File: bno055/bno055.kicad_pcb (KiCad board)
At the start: 4 copper layers, 15 parts, among them U1 BNO055, Y1 NX3215SA-32.768K-STD-MUA-14

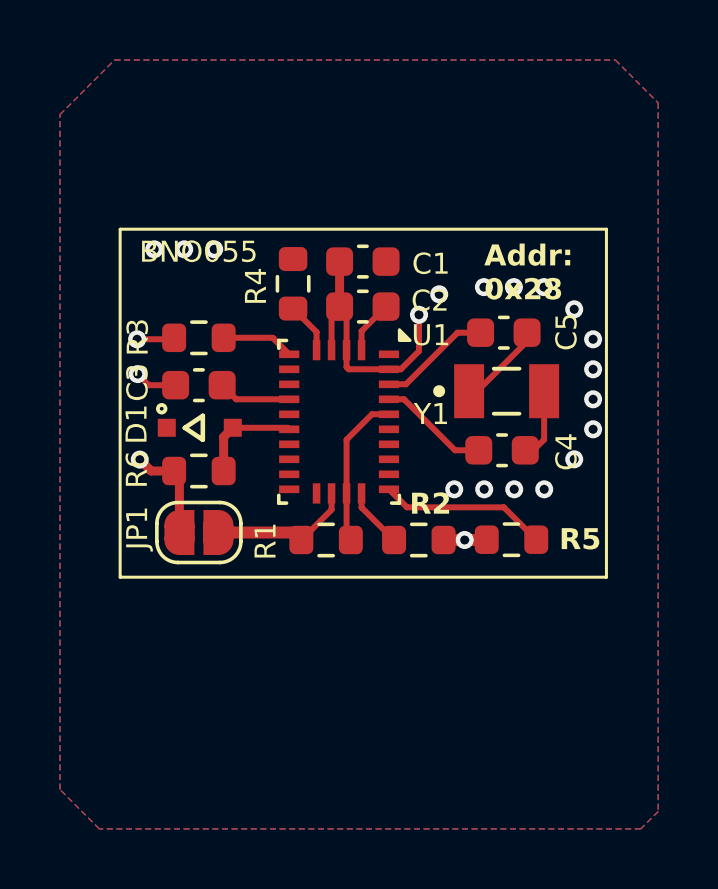
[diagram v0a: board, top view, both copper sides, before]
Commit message: fixed BNO055
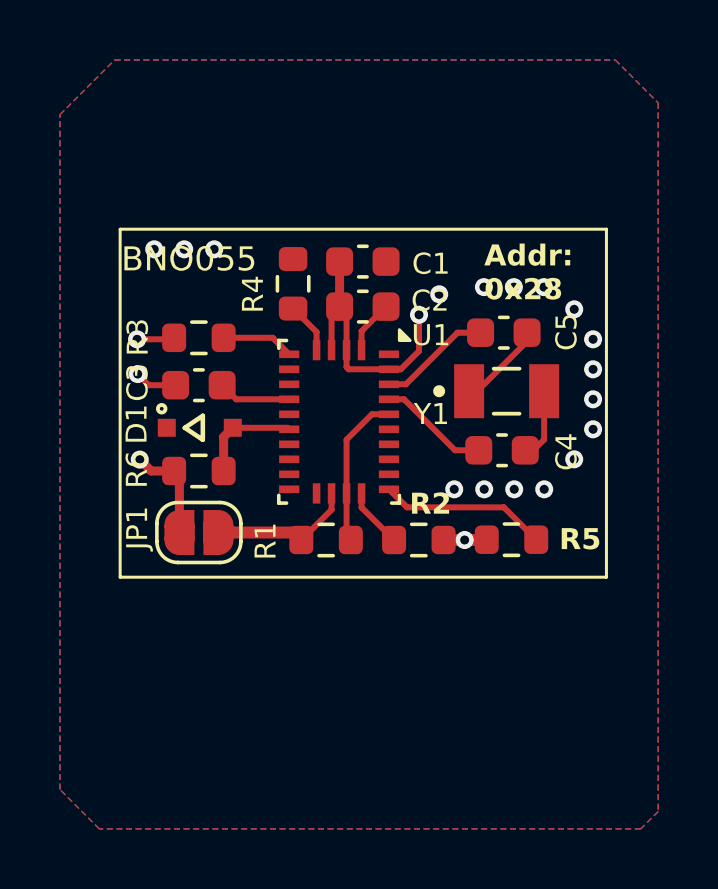
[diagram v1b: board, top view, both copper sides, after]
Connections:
- net /block_bno055/+3V3 renamed /block_bno055/3V3
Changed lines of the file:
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@@
 			(psa4output no)
 			(plot_black_and_white yes)
+			(plotinvisibletext no)
 			(sketchpadsonfab no)
 			(plotpadnumbers no)
@@
 	)
 	(net 0 "")
-	(net 1 "/block_bno055/+3V3")
+	(net 1 "/block_bno055/3V3")
 	(net 2 "/block_bno055/GND")
 	(net 3 "Net-(U1-CAP)")
@@
 			(layers "F.Cu" "F.Mask" "F.Paste")
 			(roundrect_rratio 0.25)
-			(net 1 "/block_bno055/+3V3")
+			(net 1 "/block_bno055/3V3")
 			(pintype "passive")
 		)
@@
 			(layers "F.Cu" "F.Mask" "F.Paste")
 			(roundrect_rratio 0.25)
-			(net 1 "/block_bno055/+3V3")
+			(net 1 "/block_bno055/3V3")
 			(pintype "passive")
 		)
@@
 			(size 0.254 0.675)
 			(layers "F.Cu" "F.Mask" "F.Paste")
-			(net 1 "/block_bno055/+3V3")
+			(net 1 "/block_bno055/3V3")
 			(pinfunction "VDD")
 			(pintype "power_in")
@@
 			(size 0.254 0.675)
 			(layers "F.Cu" "F.Mask" "F.Paste")
-			(net 1 "/block_bno055/+3V3")
+			(net 1 "/block_bno055/3V3")
 			(pinfunction "~{BOOT_LOAD_PIN}")
 			(pintype "input")
@@
 			(size 0.254 0.675)
 			(layers "F.Cu" "F.Mask" "F.Paste")
-			(net 1 "/block_bno055/+3V3")
+			(net 1 "/block_bno055/3V3")
 			(pinfunction "VDDIO")
 			(pintype "power_in")
@@
 			(layers "F.Cu" "F.Mask" "F.Paste")
 			(roundrect_rratio 0.25)
-			(net 1 "/block_bno055/+3V3")
+			(net 1 "/block_bno055/3V3")
 			(pintype "passive")
 		)
@@
 			(layers "F.Cu" "F.Mask" "F.Paste")
 			(roundrect_rratio 0.25)
-			(net 1 "/block_bno055/+3V3")
+			(net 1 "/block_bno055/3V3")
 			(pintype "passive")
 		)
@@
 			(layers "F.Cu" "F.Mask" "F.Paste")
 			(roundrect_rratio 0.25)
-			(net 1 "/block_bno055/+3V3")
+			(net 1 "/block_bno055/3V3")
 			(pintype "passive")
 		)
@@
 			(size 1 0.5)
 			(layers "F.Cu" "F.Mask")
-			(net 1 "/block_bno055/+3V3")
+			(net 1 "/block_bno055/3V3")
 			(pinfunction "A")
 			(pintype "passive")
@@
 		(tags "resistor")
 		(property "Reference" "R4"
-			(at -0.09 -1.23 90)
+			(at -0.35 -1.33 90)
 			(layer "F.SilkS")
 			(effects
@@
 	)
 	(gr_text "BNO055"
-		(at 104.5 69.5 0)
+		(at 103.9 69.8 0)
 		(layer "F.SilkS")
 		(effects
 			(font
-				(size 0.7 0.7)
+				(size 0.8 0.8)
 				(thickness 0.15)
 			)
@@
 	(zone
 		(net 1)
-		(net_name "/block_bno055/+3V3")
+		(net_name "/block_bno055/3V3")
 		(layer "In2.Cu")
 		(hatch edge 0.5)
